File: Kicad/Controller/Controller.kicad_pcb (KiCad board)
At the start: 2 copper layers, 4 parts, among them J1 Conn_01x07_Female, J2 Conn_01x07_Female

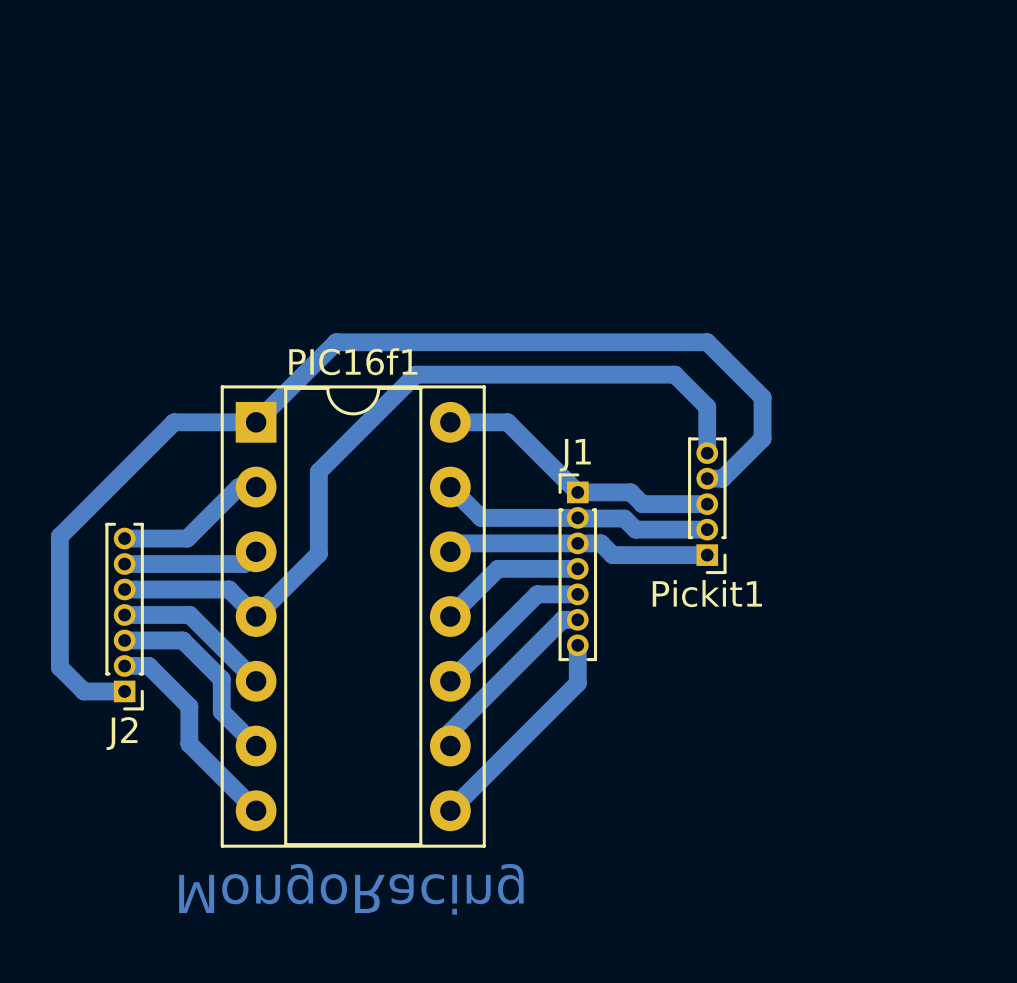
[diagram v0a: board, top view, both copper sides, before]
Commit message: h
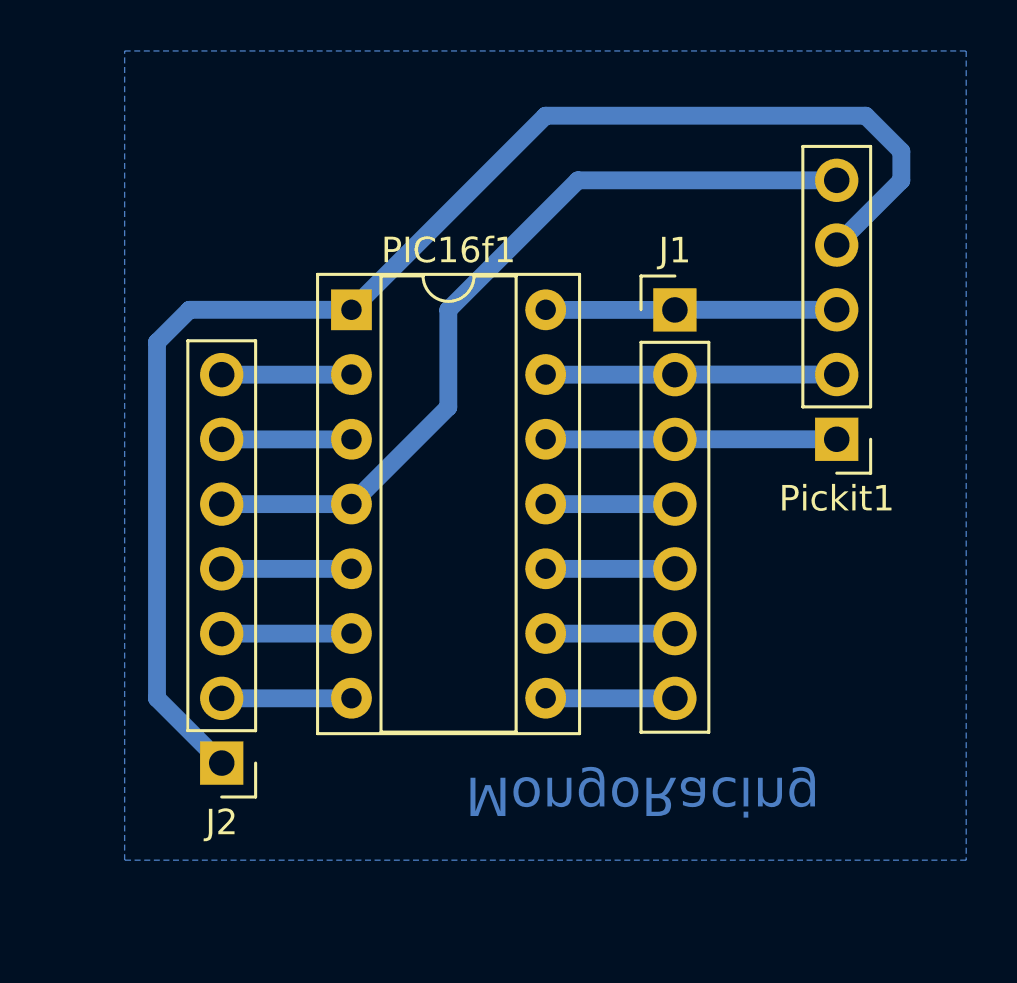
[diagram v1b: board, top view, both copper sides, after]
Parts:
- J1, J2: footprint Connector_PinHeader_1.00mm:PinHeader_1x07_P1.00mm_Vertical -> Connector_PinHeader_2.54mm:PinHeader_1x07_P2.54mm_Vertical
- Pickit1: footprint Connector_PinHeader_1.00mm:PinHeader_1x05_P1.00mm_Vertical -> Connector_PinHeader_2.54mm:PinHeader_1x05_P2.54mm_Vertical
- moved J1 8.11 mm to (135.9, 92.7)
- moved Pickit1 6.82 mm to (142.2, 97.8)
- moved PIC16f1 5.79 mm to (123.2, 92.7)
- moved J2 4.73 mm to (118.1, 110.5)
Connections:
- net Net-(J1-Pad1) renamed Earth
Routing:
- net Net-(J2-Pad1): track 44.1 -> 55.8 mm
- net Net-(J1-Pad7): track 8.56 -> 5.07 mm
- net Net-(J2-Pad2): track 8.37 -> 5.09 mm
- net Net-(J2-Pad3): track 7.62 -> 5.09 mm
- net Net-(J1-Pad6): track 7.37 -> 5.07 mm
- net Net-(J1-Pad5): track 6.41 -> 5.07 mm
- net Net-(J2-Pad4): track 6.24 -> 5.09 mm
- net Net-(J1-Pad3): track 10.4 -> 11.4 mm
- net Net-(J2-Pad7): track 6.00 -> 5.09 mm
- net Net-(J1-Pad4): track 5.77 -> 5.07 mm
- net Net-(J1-Pad2): track 10.8 -> 11.4 mm
- added copper zone on B.Cu, net Earth
